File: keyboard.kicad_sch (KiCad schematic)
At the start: 352 parts, among them J1 USB_B_Micro, J2 Conn_01x06, J3 USB_C_Receptacle_USB2.0, K0 KEYSW, K1 KEYSW, K10 KEYSW, K100 KEYSW, K101 KEYSW, K102 KEYSW, K103 KEYSW, K104 KEYSW, K105 KEYSW, K106 KEYSW, K107 KEYSW, K108 KEYSW, K11 KEYSW, K12 KEYSW, K13 KEYSW, K14 KEYSW, K15 KEYSW, K16 KEYSW, K17 KEYSW, K18 KEYSW, K19 KEYSW, K2 KEYSW, K20 KEYSW, K21 KEYSW, K22 KEYSW, K23 KEYSW, K24 KEYSW, K25 KEYSW, K26 KEYSW, K27 KEYSW, K28 KEYSW, K29 KEYSW, K3 KEYSW, K30 KEYSW, K31 KEYSW, K32 KEYSW, K33 KEYSW, K34 KEYSW, K35 KEYSW, K36 KEYSW, K37 KEYSW, K38 KEYSW, K39 KEYSW, K4 KEYSW, K40 KEYSW, K41 KEYSW, K42 KEYSW, K43 KEYSW, K44 KEYSW, K45 KEYSW, K46 KEYSW, K47 KEYSW, K48 KEYSW, K49 KEYSW, K5 KEYSW, K50 KEYSW, K51 KEYSW, K52 KEYSW, K53 KEYSW, K54 KEYSW, K55 KEYSW, K56 KEYSW, K57 KEYSW, K58 KEYSW, K59 KEYSW, K6 KEYSW, K60 KEYSW, K61 KEYSW, K62 KEYSW, K63 KEYSW, K64 KEYSW, K65 KEYSW, K66 KEYSW, K67 KEYSW, K68 KEYSW, K69 KEYSW, K7 KEYSW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

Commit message: pcb almost done
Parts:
- removed J1: USB_B_Micro, Connector_USB:USB_Micro-B_Wuerth_629105150521_CircularHoles, symbol Connector:USB_B_Micro
- added C9: 0.1u, Capacitor_SMD:C_0805_2012Metric_Pad1.15x1.40mm_HandSolder, symbol Device:C
- added F1: Fuse, Fuse:Fuse_1206_3216Metric_Pad1.42x1.75mm_HandSolder, symbol Device:Fuse
- added JP3: Jumper_2_Open, Jumper:SolderJumper-2_P1.3mm_Open_Pad1.0x1.5mm, symbol Jumper:Jumper_2_Open
- added JP4: SolderJumper_3_Open, Jumper:SolderJumper-3_P1.3mm_Open_RoundedPad1.0x1.5mm, symbol Jumper:SolderJumper_3_Open
- added Q1: Q_PMOS_DGS, Package_TO_SOT_SMD:ATPAK-2, symbol Device:Q_PMOS_DSG
- added Q2: Q_NMOS_DGS, Package_TO_SOT_SMD:SOT-23, symbol Device:Q_NMOS_DSG
- added R1, R4: 5.11k, Resistor_SMD:R_0805_2012Metric_Pad1.20x1.40mm_HandSolder, symbol Device:R
- added R5: 1M, Resistor_SMD:R_0805_2012Metric_Pad1.20x1.40mm_HandSolder, symbol Device:R
- added R6: 10k, Resistor_SMD:R_0805_2012Metric_Pad1.20x1.40mm_HandSolder, symbol Device:R
- added R7: 220k, Resistor_SMD:R_0805_2012Metric_Pad1.20x1.40mm_HandSolder, symbol Device:R
- added X1: ASE-xxxMHz, Oscillator:Oscillator_SMD_Abracon_ASE-4Pin_3.2x2.5mm, symbol Oscillator:ASE-xxxMHz
- C6, C7, C8: footprint Capacitor_SMD:C_0805_2012Metric_Pad1.15x1.40mm_HandSolder -> Capacitor_SMD:C_0805_2012Metric_Pad1.18x1.45mm_HandSolder
- J2: footprint Connector_PinHeader_2.54mm:PinHeader_1x06_P2.54mm_Vertical -> Connector_PinHeader_1.27mm:PinHeader_1x06_P1.27mm_Vertical
- J3: footprint (none) -> Connector_USB:USB_C_Receptacle_GCT_USB4085
- renumbered D189 to D275, D198 to D276, D209 to D277, D116 to D278, D121 to D279, D127 to D280, D132 to D281, D137 to D282, D142 to D283, D146 to D284, D152 to D285, D157 to D286, D162 to D287, D168 to D288, D174 to D289, D181 to D290, D205 to D291, D191 to D292, D201 to D293, D212 to D294, D220 to D295, D114 to D296, D119 to D297, D125 to D298, D149 to D299, D165 to D300, D170 to D301, D176 to D302, D183 to D303, D193 to D304, D202 to D305, D213 to D306, D192 to D307, D204 to D308
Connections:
- net Col_0: now also U1.20 (PA4); no longer U1.4 (PC15)
- net Col_1: now also U1.21 (PA5); no longer U1.3 (PC14)
- net GND: now also D110.2 (VSS), D111.2 (VSS), D112.2 (VSS), D200.2 (VSS), D201.2 (VSS), D202.2 (VSS), D203.2 (VSS), D204.2 (VSS), D205.2 (VSS), D206.2 (VSS), D207.2 (VSS), D208.2 (VSS), D209.2 (VSS), D210.2 (VSS), D211.2 (VSS), D212.2 (VSS), D213.2 (VSS), D214.2 (VSS), D215.2 (VSS), D216.2 (VSS), D217.2 (VSS), D218.2 (VSS), D219.2 (VSS), D220.2 (VSS), D221.2 (VSS), D222.2 (VSS), D223.2 (VSS), D224.2 (VSS), D225.2 (VSS), D226.2 (VSS), D227.2 (VSS), D228.2 (VSS), D229.2 (VSS), D230.2 (VSS), D231.2 (VSS), D232.2 (VSS), D233.2 (VSS), D234.2 (VSS), D235.2 (VSS), D236.2 (VSS), D237.2 (VSS), D238.2 (VSS), D239.2 (VSS), D240.2 (VSS), D241.2 (VSS), D242.2 (VSS), D243.2 (VSS), D244.2 (VSS), D245.2 (VSS), D246.2 (VSS), D247.2 (VSS), D248.2 (VSS), D249.2 (VSS), D250.2 (VSS), D251.2 (VSS), D252.2 (VSS), D253.2 (VSS), D254.2 (VSS), D255.2 (VSS), D256.2 (VSS), D257.2 (VSS), D258.2 (VSS), D259.2 (VSS), D260.2 (VSS), D261.2 (VSS), D262.2 (VSS), D263.2 (VSS), D264.2 (VSS), D265.2 (VSS), D266.2 (VSS), D267.2 (VSS), D268.2 (VSS), D269.2 (VSS), D270.2 (VSS), D271.2 (VSS), D272.2 (VSS), D273.2 (VSS), D274.2 (VSS), D275.2 (VSS), D276.2 (VSS), D277.2 (VSS), D278.2 (VSS), D279.2 (VSS), D280.2 (VSS), D281.2 (VSS), D282.2 (VSS), D283.2 (VSS), D284.2 (VSS), D285.2 (VSS), D286.2 (VSS), D287.2 (VSS), D288.2 (VSS), D289.2 (VSS), D290.2 (VSS), D291.2 (VSS), D292.2 (VSS), D293.2 (VSS), D294.2 (VSS), D295.2 (VSS), D296.2 (VSS), D297.2 (VSS), D298.2 (VSS), D299.2 (VSS), D300.2 (VSS), D301.2 (VSS), D302.2 (VSS), D303.2 (VSS), D304.2 (VSS), D305.2 (VSS), D306.2 (VSS), D307.2 (VSS), D308.2 (VSS), J3.A1 (GND), J3.A12 (GND), J3.B1 (GND), J3.B12 (GND), C9.2, JP4.3 (B), Q2.2 (S), R1.2, R4.2, R5.1, X1.2 (GND)
- net VBUS: now also J3.A4 (VBUS), J3.A9 (VBUS), J3.B4 (VBUS), J3.B9 (VBUS), F1.1
- net VCC: now also C9.1, JP4.1 (A), X1.4 (Vdd)
- net at R2.1: now also U1.44 (PA11); no longer U1.45 (PA12)
- net at R2.2: now also J3.A7 (D-), J3.B7 (D-)
- net at R3.1: now also U1.45 (PA12); no longer U1.44 (PA11)
- net at R3.2: now also J3.A6 (D+), J3.B6 (D+)
- net at D208.1 (DOUT): now also D209.3 (DIN)
- net at D208.3 (DIN): now also D207.1 (DOUT)
- net +5V: now reaches D208.4 (VDD)
- net +5V: now also D110.4 (VDD), D111.4 (VDD), D112.4 (VDD), D200.4 (VDD), D201.4 (VDD), D202.4 (VDD), D203.4 (VDD), D204.4 (VDD), D205.4 (VDD), D206.4 (VDD), D207.4 (VDD), D209.4 (VDD), D210.4 (VDD), D211.4 (VDD), D212.4 (VDD), D213.4 (VDD), D214.4 (VDD), D215.4 (VDD), D216.4 (VDD), D217.4 (VDD), D218.4 (VDD), D219.4 (VDD), D220.4 (VDD), D221.4 (VDD), D222.4 (VDD), D223.4 (VDD), D224.4 (VDD), D225.4 (VDD), D226.4 (VDD), D227.4 (VDD), D228.4 (VDD), D229.4 (VDD), D230.4 (VDD), D231.4 (VDD), D232.4 (VDD), D233.4 (VDD), D234.4 (VDD), D235.4 (VDD), D236.4 (VDD), D237.4 (VDD), D238.4 (VDD), D239.4 (VDD), D240.4 (VDD), D241.4 (VDD), D242.4 (VDD), D243.4 (VDD), D244.4 (VDD), D245.4 (VDD), D246.4 (VDD), D247.4 (VDD), D248.4 (VDD), D249.4 (VDD), D250.4 (VDD), D251.4 (VDD), D252.4 (VDD), D253.4 (VDD), D254.4 (VDD), D255.4 (VDD), D256.4 (VDD), D257.4 (VDD), D258.4 (VDD), D259.4 (VDD), D260.4 (VDD), D261.4 (VDD), D262.4 (VDD), D263.4 (VDD), D264.4 (VDD), D265.4 (VDD), D266.4 (VDD), D267.4 (VDD), D268.4 (VDD), D269.4 (VDD), D270.4 (VDD), D271.4 (VDD), D272.4 (VDD), D273.4 (VDD), D274.4 (VDD), D275.4 (VDD), D276.4 (VDD), D277.4 (VDD), D278.4 (VDD), D279.4 (VDD), D280.4 (VDD), D281.4 (VDD), D282.4 (VDD), D283.4 (VDD), D284.4 (VDD), D285.4 (VDD), D286.4 (VDD), D287.4 (VDD), D288.4 (VDD), D289.4 (VDD), D290.4 (VDD), D291.4 (VDD), D292.4 (VDD), D293.4 (VDD), D294.4 (VDD), D295.4 (VDD), D296.4 (VDD), D297.4 (VDD), D298.4 (VDD), D299.4 (VDD), D300.4 (VDD), D301.4 (VDD), D302.4 (VDD), D303.4 (VDD), D304.4 (VDD), D305.4 (VDD), D306.4 (VDD), D307.4 (VDD), D308.4 (VDD), JP3.1 (A), Q1.1 (D)
- net at D253.1 (DOUT): now also D254.3 (DIN)
- net at D253.3 (DIN): now also D252.1 (DOUT)
- net at D259.1 (DOUT): now also D260.3 (DIN)
- net at D259.3 (DIN): now also D258.1 (DOUT)
- net at D302.1 (DOUT): now also D301.3 (DIN)
- net at D302.3 (DIN): now also D303.1 (DOUT)
- net at D241.1 (DOUT): now also D242.3 (DIN)
- net at D241.3 (DIN): now also D220.1 (DOUT)
- net at D303.3 (DIN): now also D304.1 (DOUT)
- net at D256.1 (DOUT): now also D257.3 (DIN)
- net at D256.3 (DIN): now also D255.1 (DOUT)
- net at D267.1 (DOUT): now also D266.3 (DIN)
- net at D267.3 (DIN): now also D268.1 (DOUT)
- net at D301.1 (DOUT): now also D300.3 (DIN)
- net at D295.1 (DOUT): now also D308.3 (DIN)
- net at D295.3 (DIN): now also D294.1 (DOUT)
- net at D220.3 (DIN): now also D221.1 (DOUT)
- net at D299.1 (DOUT): now also D298.3 (DIN)
- net at D299.3 (DIN): now also D300.1 (DOUT)
- net at D110.1 (DOUT): now also D274.3 (DIN)
- net at D110.3 (DIN): now also D111.1 (DOUT)
- net at D269.1 (DOUT): now also D268.3 (DIN)
- net at D269.3 (DIN): now also D270.1 (DOUT)
- net at D255.3 (DIN): now also D254.1 (DOUT)
- net at D242.1 (DOUT): now also D243.3 (DIN)
- net at D262.1 (DOUT): now also D278.3 (DIN)
- net at D262.3 (DIN): now also D263.1 (DOUT)
- net at D205.1 (DOUT): now also D206.3 (DIN)
- net at D205.3 (DIN): now also D204.1 (DOUT)
- net at D280.1 (DOUT): now also D281.3 (DIN)
- net at D280.3 (DIN): now also D279.1 (DOUT)
- net at D239.1 (DOUT): now also D238.3 (DIN)
- net at D239.3 (DIN): now also D240.1 (DOUT)
- net at D305.1 (DOUT): now also D304.3 (DIN)
- net at D305.3 (DIN): now also D306.1 (DOUT)
- net at D224.1 (DOUT): now also D223.3 (DIN)
- net at D224.3 (DIN): now also D225.1 (DOUT)
- net at D237.1 (DOUT): now also D236.3 (DIN)
- net at D237.3 (DIN): now also D238.1 (DOUT)
- net at D216.1 (DOUT): now also D217.3 (DIN)
- net at D216.3 (DIN): now also D215.1 (DOUT)
- net at D229.1 (DOUT): now also D228.3 (DIN)
- net at D229.3 (DIN): now also D230.1 (DOUT)
- net at D293.1 (DOUT): now also D294.3 (DIN)
- net at D293.3 (DIN): now also D292.1 (DOUT)
- net at D289.1 (DOUT): now also D290.3 (DIN)
- net at D289.3 (DIN): now also D288.1 (DOUT)
- net at D281.1 (DOUT): now also D282.3 (DIN)
- net D_LED: now reaches U1.41 (PA8)
- net D_LED: now also D200.3 (DIN)
- net LED_EN: now reaches U1.61 (PB8)
- net LED_EN: now also R7.1
- net at D230.3 (DIN): now also D231.1 (DOUT)
- net at D286.1 (DOUT): now also D287.3 (DIN)
- net at D286.3 (DIN): now also D285.1 (DOUT)
- net at D235.1 (DOUT): now also D234.3 (DIN)
- net at D235.3 (DIN): now also D236.1 (DOUT)
- net at D243.1 (DOUT): now also D244.3 (DIN)
- net at D307.1 (DOUT): now also D306.3 (DIN)
- net at D307.3 (DIN): now also D308.1 (DOUT)
- net at D257.1 (DOUT): now also D258.3 (DIN)
- net at D225.3 (DIN): now also D226.1 (DOUT)
- net at D251.1 (DOUT): now also D252.3 (DIN)
- net at D251.3 (DIN): now also D250.1 (DOUT)
- net at D273.1 (DOUT): now also D272.3 (DIN)
- net at D273.3 (DIN): now also D274.1 (DOUT)
- net at D203.1 (DOUT): now also D204.3 (DIN)
- net at D203.3 (DIN): now also D202.1 (DOUT)
- net at D232.1 (DOUT): now also D231.3 (DIN)
- net at D232.3 (DIN): now also D233.1 (DOUT)
- net at D233.3 (DIN): now also D234.1 (DOUT)
- net at D275.1 (DOUT): now also D112.3 (DIN)
- net at D275.3 (DIN): now also D276.1 (DOUT)
- net at D284.1 (DOUT): now also D285.3 (DIN)
- net at D284.3 (DIN): now also D283.1 (DOUT)
- net at J3.A5 (CC1): now also R4.1
- net at J3.B5 (CC2): now also R1.1
- net at J3.S1 (SHIELD): now also R5.2
- net at D290.1 (DOUT): now also D291.3 (DIN)
- net at D297.1 (DOUT): now also D296.3 (DIN)
- net at D297.3 (DIN): now also D298.1 (DOUT)
- net at D282.1 (DOUT): now also D283.3 (DIN)
- net at D211.1 (DOUT): now also D212.3 (DIN)
- net at D211.3 (DIN): now also D210.1 (DOUT)
- net at D248.1 (DOUT): now also D249.3 (DIN)
- net at D248.3 (DIN): now also D247.1 (DOUT)
- net at D218.1 (DOUT): now also D219.3 (DIN)
- net at D218.3 (DIN): now also D217.1 (DOUT)
- net at D221.3 (DIN): now also D222.1 (DOUT)
- net at D201.1 (DOUT): now also D202.3 (DIN)
- net at D201.3 (DIN): now also D200.1 (DOUT)
- net at D291.1 (DOUT): now also D292.3 (DIN)
- net at D223.1 (DOUT): now also D222.3 (DIN)
- net at D215.3 (DIN): now also D214.1 (DOUT)
- net at D276.3 (DIN): now also D277.1 (DOUT)
- net at D249.1 (DOUT): now also D250.3 (DIN)
- net at D288.3 (DIN): now also D287.1 (DOUT)
- net at D213.1 (DOUT): now also D214.3 (DIN)
- net at D213.3 (DIN): now also D212.1 (DOUT)
- net at D226.3 (DIN): now also D227.1 (DOUT)
- net at D272.1 (DOUT): now also D271.3 (DIN)
- net at D111.3 (DIN): now also D112.1 (DOUT)
- net at D264.1 (DOUT): now also D263.3 (DIN)
- net at D264.3 (DIN): now also D265.1 (DOUT)
- net at D266.1 (DOUT): now also D265.3 (DIN)
- net at D207.3 (DIN): now also D206.1 (DOUT)
- net at D260.1 (DOUT): now also D261.3 (DIN)
- net at D247.3 (DIN): now also D246.1 (DOUT)
- net at D227.3 (DIN): now also D228.1 (DOUT)
- net at D240.3 (DIN): now also D219.1 (DOUT)
- net at D209.1 (DOUT): now also D210.3 (DIN)
- net at D279.3 (DIN): now also D278.1 (DOUT)
- net at D245.1 (DOUT): now also D246.3 (DIN)
- net at D245.3 (DIN): now also D244.1 (DOUT)
- net at D261.1 (DOUT): now also D277.3 (DIN)
- net at D270.3 (DIN): now also D271.1 (DOUT)
- new net: Q1.3 (G), Q2.1 (D), R6.1
- new net: JP4.2 (C), X1.1 (EN)
- new net: U1.3 (PC14), X1.3 (OUT)
- new net: Q2.3 (G), R7.2
- new net Vfuse: F1.2, JP3.2 (B), Q1.2 (S), R6.2
- no-connect marks 1 -> 3
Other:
- moved on the sheet: C1, C2, C3, C4, C5, C6, C7, C8, D110, D111, D112, D200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

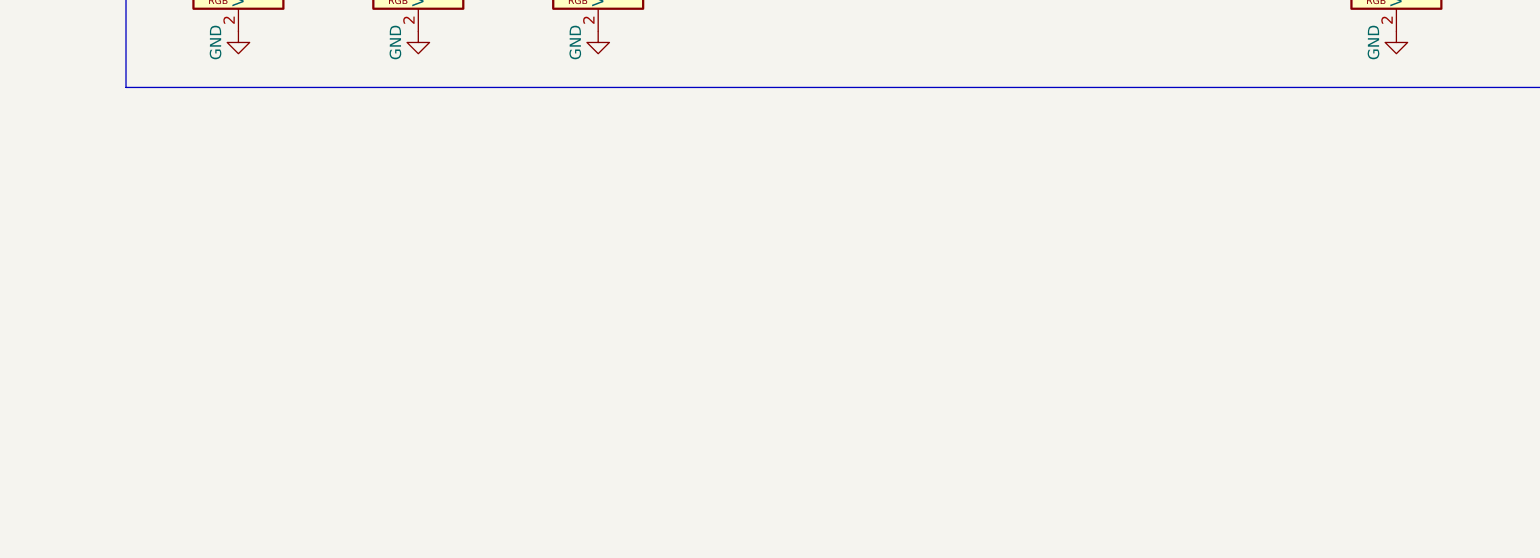
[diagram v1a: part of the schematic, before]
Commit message: PCB finished
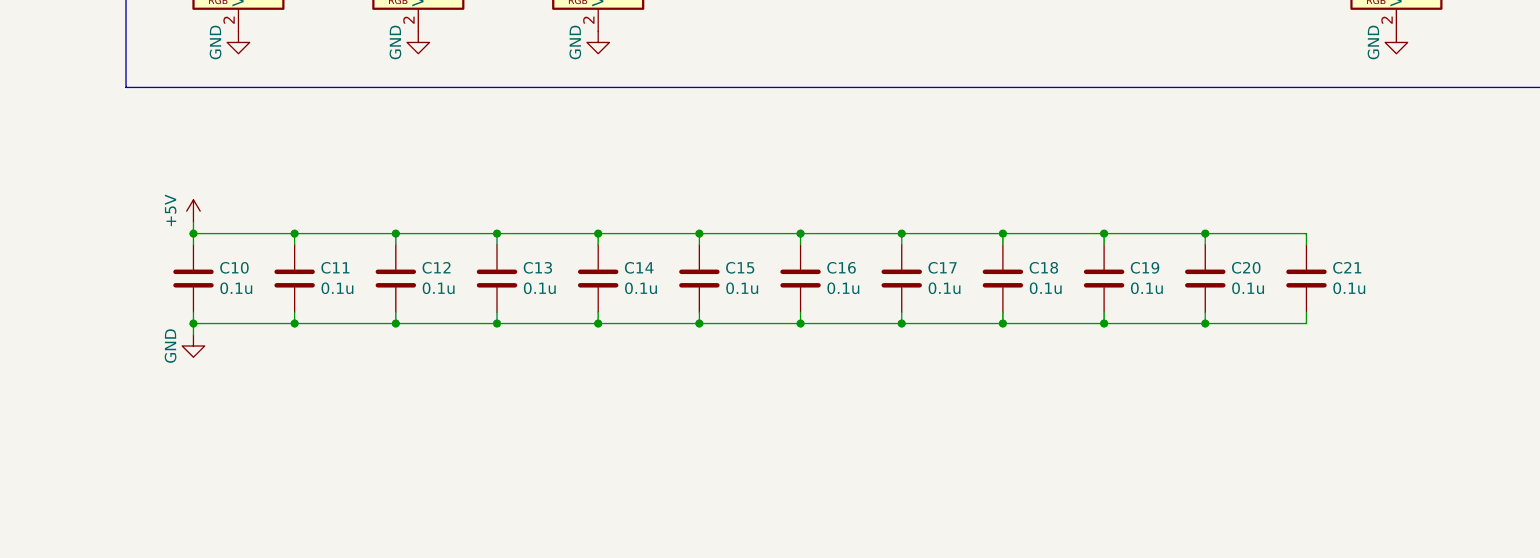
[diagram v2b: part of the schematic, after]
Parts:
- added C10, C11, C12, C13, C14, C15, C16, C17, C18, C19, C20, C21: 0.1u, Capacitor_SMD:C_0805_2012Metric_Pad1.18x1.45mm_HandSolder, symbol Device:C
- C9: footprint Capacitor_SMD:C_0805_2012Metric_Pad1.15x1.40mm_HandSolder -> Capacitor_SMD:C_0805_2012Metric_Pad1.18x1.45mm_HandSolder
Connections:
- net +5V: now also C10.1, C11.1, C12.1, C13.1, C14.1, C15.1, C16.1, C17.1, C18.1, C19.1, C20.1, C21.1
- net GND: now also C10.2, C11.2, C12.2, C13.2, C14.2, C15.2, C16.2, C17.2, C18.2, C19.2, C20.2, C21.2
